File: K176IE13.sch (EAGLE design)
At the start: 104 parts, among them J1 0R-JUMPB

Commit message: .
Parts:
- added C15, C16: 22n, rcl:C-EUC1206
- added C19: 120, rcl:C-EUC0805
- added C20, C21, C24: 100n, rcl:C-EUC0805
- added C22: 100m, rcl:CPOL-EUE2.5-5
- added C23: 470m, rcl:CPOL-EUE3.5-8
- added C25, C26: 33, rcl:C-EU025-025X050
- added C27: 2n2, rcl:C-EU025-025X050
- added C28, C29: 100m, rcl:CPOL-EUE2-5
- added C30: 1m, rcl:C-EU025-025X050
- added D10, D11: (no value), diode:DIODE-SOD80C
- added D12: (no value), diode:ZENER-DIODEDO34-7
- added DA1: MC34063AD, mc34063-2:MC34063AD
- added DA4: LM311,К554СА3KY, IC:LM311,К554СА3KY
- added IV1, IV2, IV3, IV6: 24r, rcl:R-EU_M0805
- added IV3A: 17r, rcl:R-EU_M0805
- added L4, L6, L7: (no value), rcl:L-USL3225M
- added L8, L9: 50mkhn, rcl:L-USTFI0305
- added R: (no value), rcl:R-EU_M0805
- added R19, R33: 100k, rcl:R-EU_M0805
- added R20, R21: 56k, rcl:R-EU_M0805
- added R22, R23: 8k2, rcl:R-EU_M0805
- added R26: 180, rcl:R-EU_M0805
- added R30: 0.33r, rcl:R-EU_M1206
- added R31: 470, rcl:R-EU_M0805
- added R32: 1k, rcl:R-EU_M0805
- added R34, R35: 47k, rcl:R-EU_0207/10
- added R36: 1k, rcl:R-EU_0207/10
- added R37: 30k, rcl:R-EU_0207/10
- added R38, R39, R40: 15k, rcl:R-EU_0207/10
- added R41, R42: 220, rcl:R-EU_0207/10
- added R43: 10k, rcl:R-EU_0207/10
- added VT10, VT8: BJT_NPN_TO-92_CBE, m_transistor:BJT_NPN_TO-92_CBE
- added VT11, VT9: BJT_PNP_TO-92_CBE, m_transistor:BJT_PNP_TO-92_CBE
- added VT2, VT7: (no value), m_transistor:MOSFET-N_DPACK
- added VT3, VT5: КТ3102, transistor-npn:BC338
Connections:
- new net -24V: C30.1, D12.A
- new net N$100: IV3A.2, R.1
- new net N$101: C28.+, R37.2, R38.2, VT10.E, VT11.E
- new net N$102: C25.2, C26.1, DA4.OUT, R34.1, R35.2, R36.1
- new net N$103: C25.1, R34.2, VT9.B
- new net N$104: C26.2, R35.1, VT8.B
- new net N$105: C30.2, D12.C, R41.1, R42.2, R43.2
- new net N$106: C28.-, R41.2
- new net N$107: C29.-, R42.1
- new net N$109: DA4.-IN, R37.1, R39.2, R40.1
- new net N$110: C27.1, DA4.+IN, R38.1
- new net N$28: C16.1, L4.2, VT5.C
- new net N$69: R19.1, VT2.G
- new net N$70: C203.2, DA2.GND, DA2.SWE, VT2.D
- new net N$71: C15.2, L6.1, VT3.C
- new net N$72: R20.1, R22.1, VT5.B
- new net N$73: R21.1, R23.1, VT3.B
- new net N$74: DA1.DC, R26.2
- new net N$75: L4.1, L6.2, R22.2, R23.2
- new net N$76: C16.2, R21.2
- new net N$78: DA1.IS, L8.1, R26.1, R30.2
- new net N$80: C15.1, R20.2
- new net N$83: VT10.B, VT11.B, VT8.C, VT9.C
- new net N$87: C19.1, DA1.TC
- new net N$89: C24.1, DA1.FB, R31.1, R32.2
- new net N$90: D10.A, L9.2
- new net N$95: R33.1, VT7.G
- new net N$96: C20.2, C22.-, D11.C, IV1.1, IV2.1, IV3.1, IV3A.1, IV6.1
- new net N$97: D10.C, R31.2
- new net N$99: C20.1, C22.+, DA1.SWC, IV1.2, IV2.2, IV3.2, IV6.2, L8.2, L9.1, R.2
- new net V+: DA4.V+, R36.2, R40.2, VT10.C, VT9.E
- net +3V3: now also C21.1, C23.+, DA1.VCC, R30.1
- net GND: now also C19.2, C21.2, C23.-, C24.2, C27.2, C29.+, D11.A, DA1.GND, DA1.SWE, DA4.GND, DA4.V-, R19.2, R32.1, R33.2, R39.1, R43.1, VT11.C, VT2.S, VT3.E, VT5.E, VT7.S, VT8.E; no longer C203.2, DA2.GND, DA2.SWE
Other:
- note added: "1.25в"
- note added: "1.8в"
- moved on the sheet: C201, C202, C203, C204, C205, DA2, JP6, JP7, L201, R201, R202, R203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

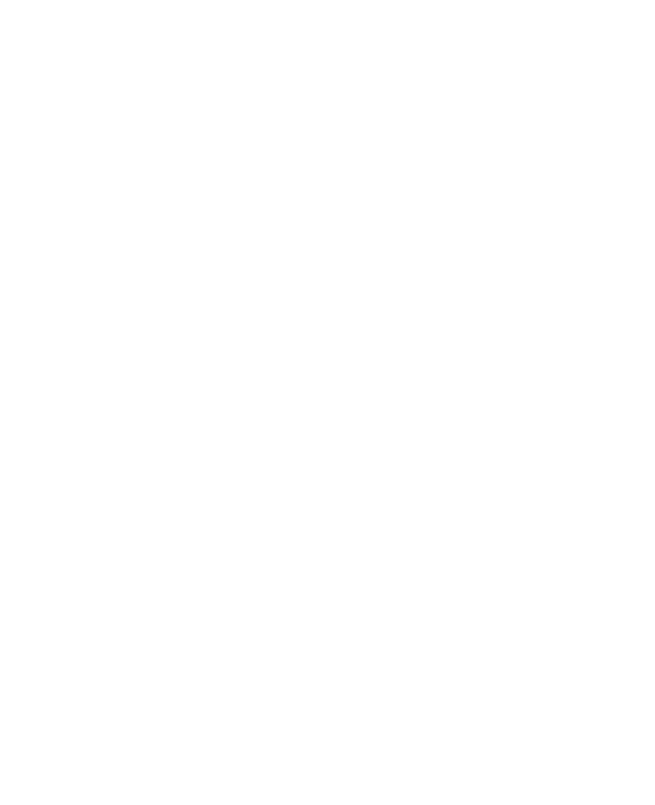
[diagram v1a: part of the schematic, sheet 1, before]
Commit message: .
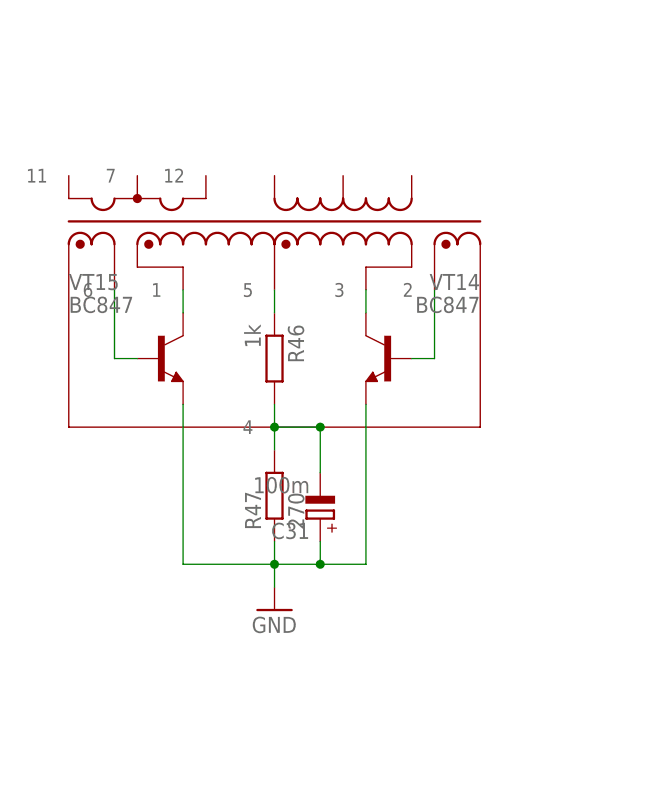
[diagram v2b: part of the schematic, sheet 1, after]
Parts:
- added C31: 100m, rcl:CPOL-EUE2-5
- added R46: 1k, rcl:R-EU_M0805
- added R47: 270, rcl:R-EU_M0805
- added U$24: TRAN_EE16, ie13:TRAN_EE16
- added VT14, VT15: BC847, m_transistor:BJT_NPN_SOT23_BCE
- R36, R39: device rcl:R-EU_0207/10 -> rcl:R-EU_M0805
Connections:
- new net N$116: U$24.1, VT15.C
- new net N$117: U$24.3, VT14.C
- new net N$118: U$24.2, VT14.B
- new net N$119: U$24.6, VT15.B
- new net N$120: R46.1, U$24.5
- new net N$121: C31.-, R46.2, R47.2, U$24.4
- net GND: now also C31.+, R47.1, VT14.E, VT15.E
